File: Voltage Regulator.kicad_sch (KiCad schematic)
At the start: 4 parts, among them U4 AP2112K-3.3TRG1

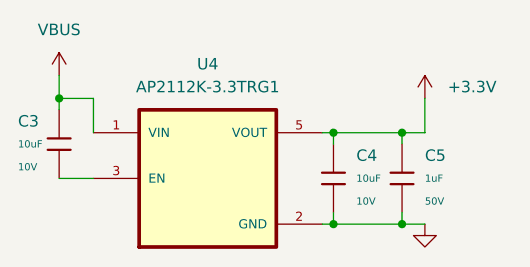
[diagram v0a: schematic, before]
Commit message: feat: Preserve saved puck design and fabrication package
Original-author: Zachariah K. Sharma <zachariah.sharma@gmail.com>
Source-commit: e899556739295891c68fe5bb4e4d2c3c5016f347
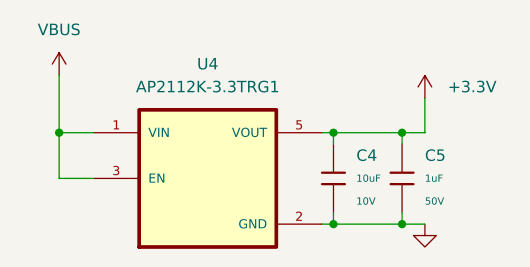
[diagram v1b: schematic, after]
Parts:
- removed C3: 10uF, PCM_JLCPCB:C_0603, symbol PCM_JLCPCB-Capacitors:0603,10uF
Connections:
- net VBUS: now also U4.3 (EN)
